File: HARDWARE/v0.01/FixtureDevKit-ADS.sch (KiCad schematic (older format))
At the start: 41 parts

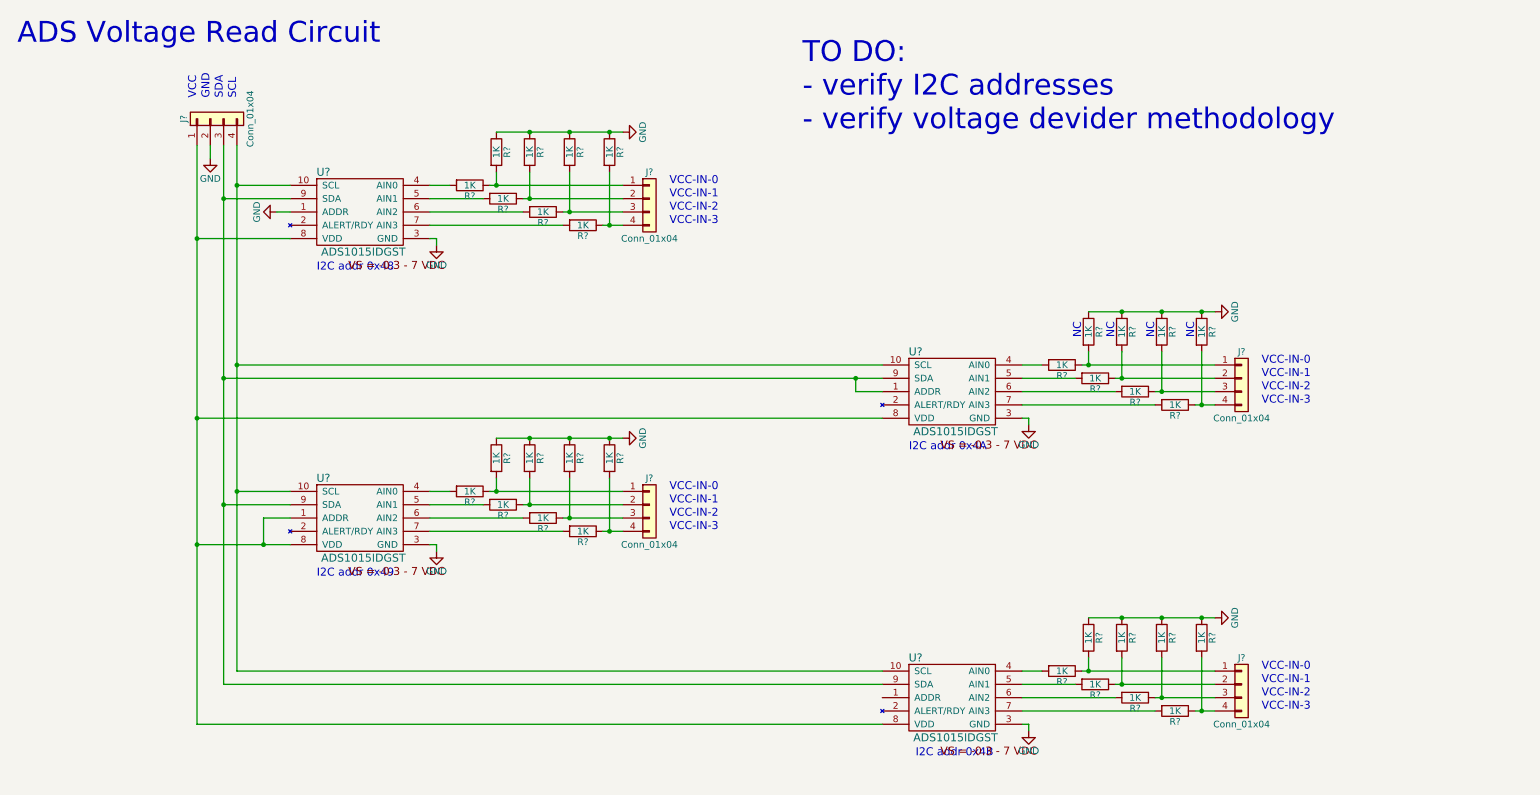
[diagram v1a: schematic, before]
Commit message: editing some files. cleaning stuff up.
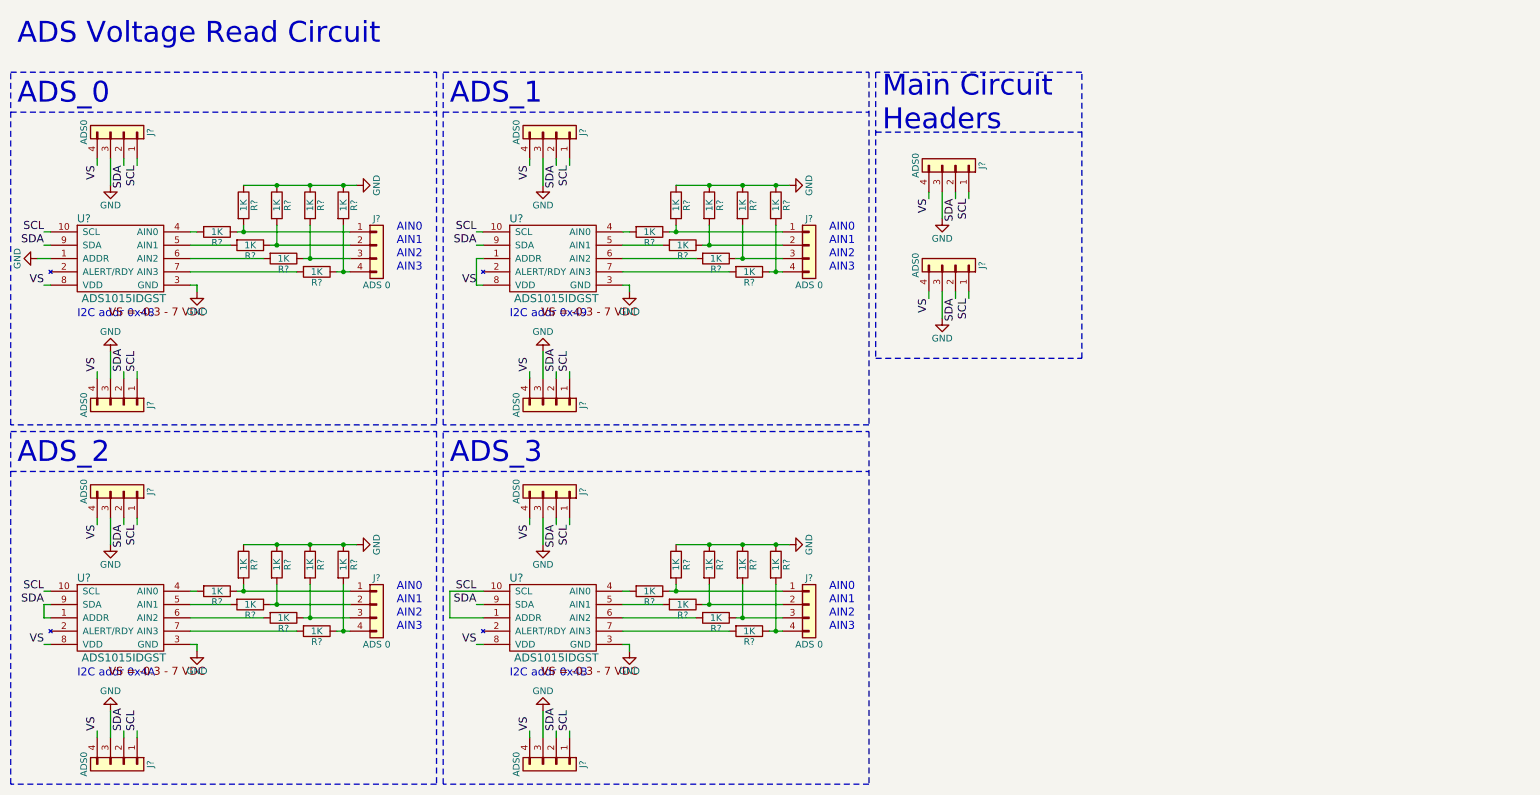
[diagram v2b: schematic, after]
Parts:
- removed J? (x5): Conn_01x04, symbol Conn_01x04
- removed R? (x32): 1K, symbol R
- removed U? (x4): ADS1015IDGST, symbol ADS1015IDGST
- added J? (x4): ADS 0, symbol Conn_01x04
- added J? (x10): ADS0, symbol Conn_01x04
- added R? (x32): 1K, symbol R
- added U? (x4): ADS1015IDGST, symbol ADS1015IDGST
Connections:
- net GND: now also J?.3 (Pin_3), J?.3 (Pin_3), J?.3 (Pin_3), J?.3 (Pin_3), J?.3 (Pin_3), J?.3 (Pin_3), J?.3 (Pin_3), J?.3 (Pin_3), J?.3 (Pin_3), J?.3 (Pin_3), R?.1, R?.1, R?.1, R?.1, R?.1, R?.1, R?.1, R?.1, R?.1, R?.1, R?.1, R?.1, R?.1, R?.1, R?.1, R?.1, U?.1 (ADDR), U?.3 (GND), U?.3 (GND), U?.3 (GND), U?.3 (GND)
- new net: R?.2, U?.4 (AIN0) (x4)
- new net: R?.2, U?.5 (AIN1) (x4)
- new net: R?.2, U?.6 (AIN2) (x4)
- new net: R?.2, U?.7 (AIN3) (x4)
- new net: J?.1 (Pin_1), R?.1, R?.2 (x4)
- new net: J?.2 (Pin_2), R?.1, R?.2 (x4)
- new net: J?.3 (Pin_3), R?.1, R?.2 (x4)
- new net: J?.4 (Pin_4), R?.1, R?.2 (x4)
- new net SCL: J?.1 (Pin_1), J?.1 (Pin_1), J?.1 (Pin_1), J?.1 (Pin_1), J?.1 (Pin_1), J?.1 (Pin_1), J?.1 (Pin_1), J?.1 (Pin_1), J?.1 (Pin_1), J?.1 (Pin_1), U?.1 (ADDR), U?.10 (SCL), U?.10 (SCL), U?.10 (SCL), U?.10 (SCL)
- new net SDA: J?.2 (Pin_2), J?.2 (Pin_2), J?.2 (Pin_2), J?.2 (Pin_2), J?.2 (Pin_2), J?.2 (Pin_2), J?.2 (Pin_2), J?.2 (Pin_2), J?.2 (Pin_2), J?.2 (Pin_2), U?.1 (ADDR), U?.9 (SDA), U?.9 (SDA), U?.9 (SDA), U?.9 (SDA)
- new net VS: J?.4 (Pin_4), J?.4 (Pin_4), J?.4 (Pin_4), J?.4 (Pin_4), J?.4 (Pin_4), J?.4 (Pin_4), J?.4 (Pin_4), J?.4 (Pin_4), J?.4 (Pin_4), J?.4 (Pin_4), U?.1 (ADDR), U?.8 (VDD), U?.8 (VDD), U?.8 (VDD), U?.8 (VDD)
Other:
- note added: "ADS_0\n"
- note added: "ADS_1"
- note added: "ADS_2"
- note added: "ADS_3"
- note added: "AIN0"
- note added: "AIN1"
- note added: "AIN2"
- note added: "AIN3"
- note added: "I2C addr 0x49"
- note added: "I2C addr 0x4A"
- note added: "Main Circuit\nHeaders"
- note removed: "GND\n"
- note removed: "I2C addr 0x49\n"
- note removed: "I2C addr 0x4A\n"
- note removed: "NC"
- note removed: "SCL"
- note removed: "SDA"
- note removed: "TO DO:\n- verify I2C addresses\n- verify voltage devider methodology"
- note removed: "VCC"
- note removed: "VCC-IN-0"
- note removed: "VCC-IN-1"
- note removed: "VCC-IN-2\n"
- note removed: "VCC-IN-3"
